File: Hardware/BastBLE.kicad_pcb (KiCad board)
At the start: 2 copper layers, 50.8 x 22.9 mm, 41 parts, among them J1 Conn_Battery, J2 SWD, J3 Conn_left, J4 Conn_right, P1 USB_C_Plug_USB2.0, Q1 DMG3415U-7, SW1 RESET, U1 AP2112K-3.3, U2 E73-2G4M08S1C, U3 MCP73831-2-OT, U4 W25Q32JVSS, Y1 32Khz

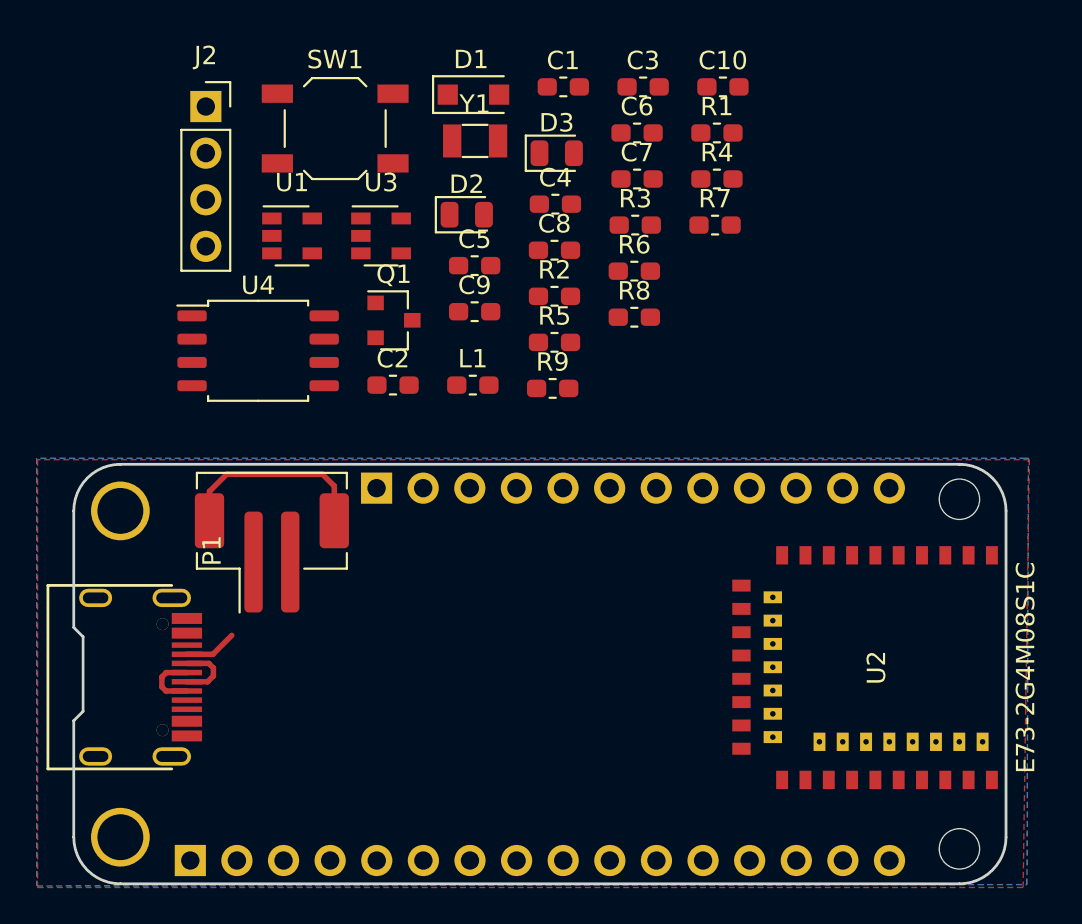
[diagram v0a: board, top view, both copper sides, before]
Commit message: fix components
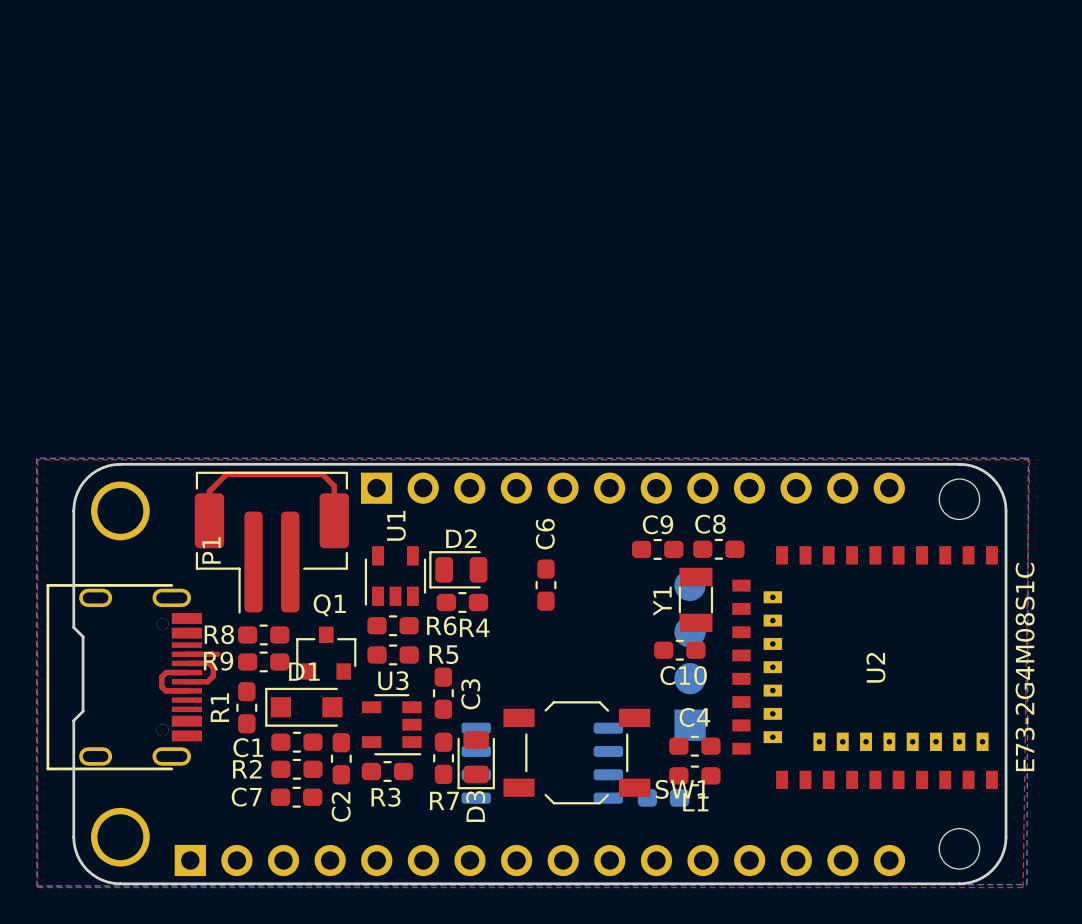
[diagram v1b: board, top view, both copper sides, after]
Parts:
- C5, J2, U4: moved to B.Cu
- moved J2 42.8 mm to (160.6, 95.5)
- moved R1 40.5 mm to (136.4, 94.5), turned to 90 degrees
- moved C1 38.5 mm to (139.2, 96.4)
- moved C7 38.5 mm to (139.1, 99.4), turned to 180 degrees
- moved SW1 36.5 mm to (154.4, 97.0)
- moved C3 34.8 mm to (147.1, 93.8), turned to 270 degrees
- moved D1 34.6 mm to (139.7, 94.5)
- moved D3 33.2 mm to (148.9, 97.2), turned to 90 degrees
- moved R3 32.7 mm to (144.1, 98.0)
- moved R7 32.6 mm to (147.2, 97.3), turned to 90 degrees
- moved C10 30.8 mm to (160.0, 91.4), turned to 180 degrees
- moved C5 30.8 mm to (159.1, 99.5)
- moved C4 30.5 mm to (160.8, 96.6)
- moved R2 29.3 mm to (139.2, 97.9)
- moved Y1 27.8 mm to (160.9, 88.7), turned to 90 degrees
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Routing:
- net Net-(P1-PadA5): track 2.87 -> 1.87 mm
